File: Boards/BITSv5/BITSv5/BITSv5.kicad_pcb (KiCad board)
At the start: 4 copper layers, 61.7 x 59.5 mm, 82 parts, among them J1 Conn_01x10_Pin, J2 USB_C_Receptacle_USB2.0, J3 Conn_01x07, J4 Conn_01x10_Pin, Q1 Q_NMOS_GSD, Q2 Q_PMOS_GSD, SW1 SW_Push, SW3 SLIDE, U1 MCU_RaspberryPi_RP2040_RP2040, U10 USBLC6-2SC6, U2 W25Q128JVS, U3 MAX-M10S, U4 MAX25255AFDA/VY+, U6 XBee_SMT, U7 TPS2121RUXR, U8 LT6703CDC-3, U9 TVS1800DRVR, Y1 12MHz

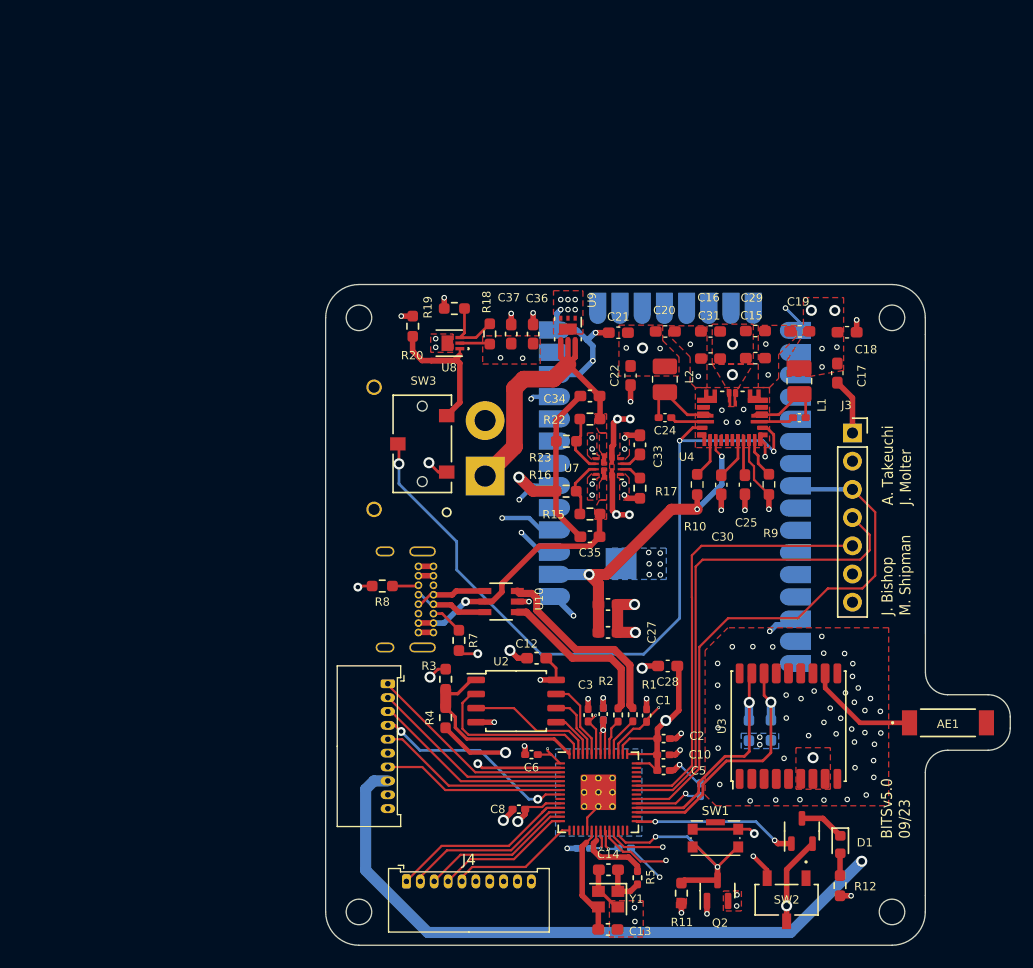
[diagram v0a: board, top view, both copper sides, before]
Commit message: bits v5 w/ dorji radio
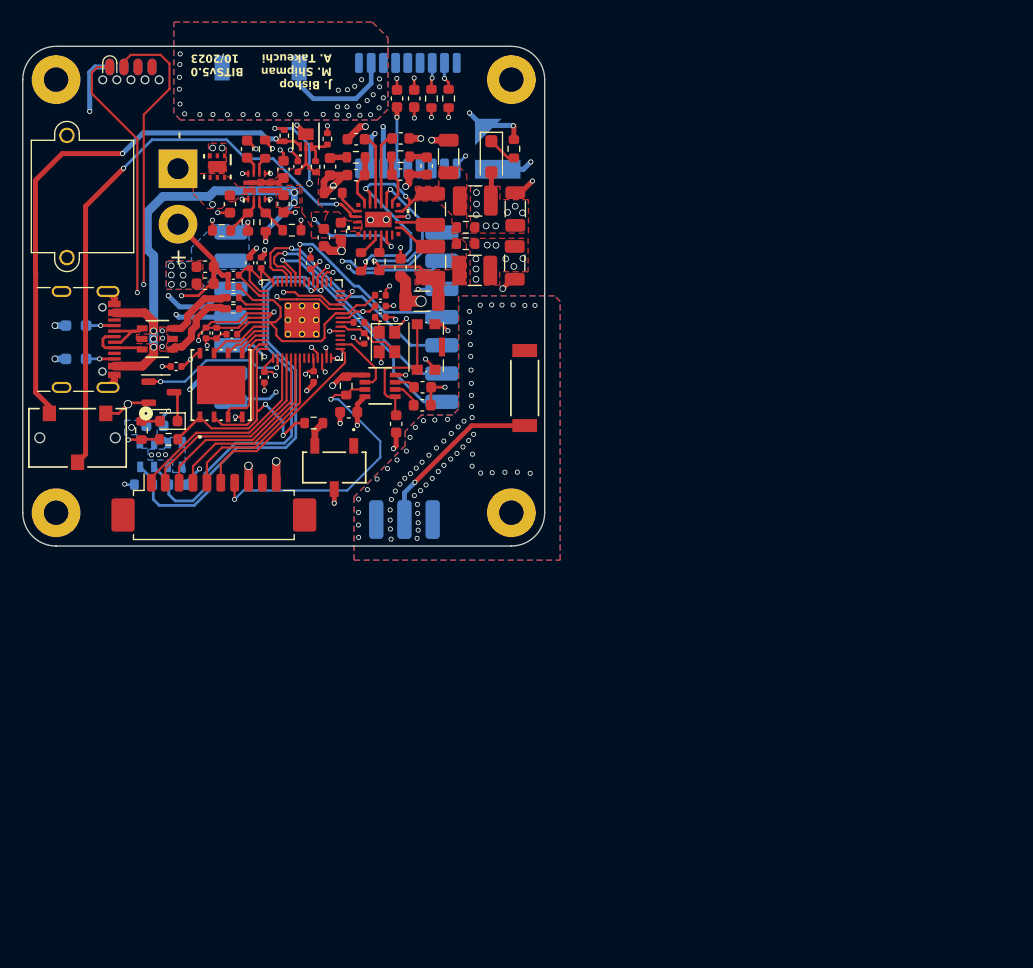
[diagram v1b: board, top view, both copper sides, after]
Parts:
- removed C31: 0.1uF, Capacitor_SMD:C_0603_1608Metric_Pad1.08x0.95mm_HandSolder
- removed J4: Conn_01x10_Pin, Connector_Molex:Molex_PicoBlade_53048-1010_1x10_P1.25mm_Horizontal
- removed Q2: Q_PMOS_GSD, Package_TO_SOT_SMD:SOT-23
- added AE2: Antenna, BITSv5:ANT_0915AT43A0026E_JOT, F.Cu at (150.4, 73.0)
- added BT2: 3V, BITSv5:SEIKO_ML414H_IV01E, B.Cu at (148.7, 51.4)
- added C38: 15uF, Capacitor_SMD:C_1206_3216Metric, F.Cu at (149.5, 61.7)
- added C39: 1uF, Capacitor_SMD:C_0603_1608Metric, F.Cu at (140.5, 46.9)
- added C40: 1uF, Capacitor_SMD:C_0603_1608Metric, F.Cu at (138.9, 46.9)
- added C41: 1uF, Capacitor_SMD:C_0603_1608Metric, F.Cu at (134.6, 75.2)
- added C42: 100nF, Capacitor_SMD:C_0603_1608Metric, F.Cu at (141.2, 74.5)
- added C43: 200nF, Capacitor_SMD:C_0603_1608Metric, F.Cu at (141.2, 72.9)
- added D2: 0.5A/40V/240mV, Diode_SMD:D_SOD-123F, F.Cu at (147.4, 52.1)
- added H1: M2, MountingHole:MountingHole_2.2mm_M2_Pad, F.Cu at (108.2, 45.2)
- added H2: M2, MountingHole:MountingHole_2.2mm_M2_Pad, F.Cu at (108.2, 84.2)
- added H3: M2, MountingHole:MountingHole_2.2mm_M2_Pad, F.Cu at (149.2, 84.2)
- added H4: M2, MountingHole:MountingHole_2.2mm_M2_Pad, F.Cu at (149.2, 45.2)
- added L3: 3.3uH, Inductor_SMD:L_1210_3225Metric, F.Cu at (146.0, 56.1)
- added L4: 3.3uH, Inductor_SMD:L_1210_3225Metric, F.Cu at (145.9, 62.4)
- added R13: 100m, Resistor_SMD:R_0603_1608Metric, F.Cu at (145.1, 60.0)
- added R14: 3.3K, Resistor_SMD:R_0603_1608Metric, F.Cu at (149.4, 51.4)
- added R27: 22.1K, Resistor_SMD:R_0603_1608Metric, F.Cu at (139.2, 52.1)
- added R29: 100K, Resistor_SMD:R_0603_1608Metric, F.Cu at (137.3, 61.6)
- added R32: 34.8K, Resistor_SMD:R_0603_1608Metric, F.Cu at (135.2, 52.2)
- added R33: 100K, Resistor_SMD:R_0603_1608Metric, F.Cu at (135.7, 61.6)
- added R34: 15K, Resistor_SMD:R_0603_1608Metric, F.Cu at (133.2, 55.4)
- added R6: 10K, Resistor_SMD:R_0603_1608Metric, B.Cu at (116.1, 81.7)
- added U11: MS5607-02BA, Package_LGA:LGA-8_3x5mm_P1.25mm, B.Cu at (117.7, 79.0)
- added U5: LT8653SIV-PBF, BITSv5:LT8653SIV-PBF, F.Cu at (137.2, 57.8)
- AE1, R7, R8, U3: moved to B.Cu
- BT1: moved to F.Cu
- C1, C10, C2, C3, C5, C6, C7, C8: footprint Capacitor_SMD:C_0402_1005Metric_Pad0.74x0.62mm_HandSolder -> Capacitor_SMD:C_0402_1005Metric
- C11, C32, C4, C9: footprint Capacitor_SMD:C_0402_1005Metric_Pad0.74x0.62mm_HandSolder -> Capacitor_SMD:C_0402_1005Metric; moved to F.Cu
- C12, C13, C14, C37: footprint Capacitor_SMD:C_0603_1608Metric_Pad1.08x0.95mm_HandSolder -> Capacitor_SMD:C_0402_1005Metric
- C15: value 0.1uF -> 4.7uF; footprint Capacitor_SMD:C_0603_1608Metric_Pad1.08x0.95mm_HandSolder -> Capacitor_SMD:C_0603_1608Metric
- C16: value 4.7uF -> 47uF; footprint Capacitor_SMD:C_0603_1608Metric_Pad1.08x0.95mm_HandSolder -> Capacitor_SMD:C_1206_3216Metric
- C17: value 22uF -> 4.7pF; footprint Capacitor_SMD:C_0603_1608Metric_Pad1.08x0.95mm_HandSolder -> Capacitor_SMD:C_0603_1608Metric
- C18, C21: value 22uF -> 470pF; footprint Capacitor_SMD:C_0603_1608Metric_Pad1.08x0.95mm_HandSolder -> Capacitor_SMD:C_0603_1608Metric
- C19: value 22uF -> 10nF; footprint Capacitor_SMD:C_0603_1608Metric_Pad1.08x0.95mm_HandSolder -> Capacitor_SMD:C_0603_1608Metric
- C20: value 22uF -> 100uF; footprint Capacitor_SMD:C_0603_1608Metric_Pad1.08x0.95mm_HandSolder -> Capacitor_SMD:C_1206_3216Metric
- C22: value 22uF -> 100nF; footprint Capacitor_SMD:C_0603_1608Metric_Pad1.08x0.95mm_HandSolder -> Capacitor_SMD:C_0603_1608Metric
- C23: value 0.1uF -> 4.7pF; footprint Capacitor_SMD:C_0402_1005Metric_Pad0.74x0.62mm_HandSolder -> Capacitor_SMD:C_0603_1608Metric
- C24: value 0.1uF -> 10nF; footprint Capacitor_SMD:C_0402_1005Metric_Pad0.74x0.62mm_HandSolder -> Capacitor_SMD:C_0603_1608Metric
- C25: value 2.2uF -> 1uF; footprint Capacitor_SMD:C_0603_1608Metric_Pad1.08x0.95mm_HandSolder -> Capacitor_SMD:C_0603_1608Metric
- C26: value 100pF -> 10uF; footprint Capacitor_SMD:C_0603_1608Metric_Pad1.08x0.95mm_HandSolder -> Capacitor_SMD:C_0603_1608Metric
- C27, C33, C34, C35, C36: footprint Capacitor_SMD:C_0603_1608Metric_Pad1.08x0.95mm_HandSolder -> Capacitor_SMD:C_0603_1608Metric
- C28: value 10uF -> 15uF; footprint Capacitor_SMD:C_0603_1608Metric_Pad1.08x0.95mm_HandSolder -> Capacitor_SMD:C_1206_3216Metric
- C29: value 4.7uF -> 100nF; footprint Capacitor_SMD:C_0603_1608Metric_Pad1.08x0.95mm_HandSolder -> Capacitor_SMD:C_0603_1608Metric; moved to B.Cu
- C30: value 4.7uF -> 100nF; footprint Capacitor_SMD:C_0603_1608Metric_Pad1.08x0.95mm_HandSolder -> Capacitor_SMD:C_0603_1608Metric
- J1: footprint Connector_Molex:Molex_PicoBlade_53048-1010_1x10_P1.25mm_Horizontal -> Connector_Molex:Molex_PicoBlade_53261-1071_1x10-1MP_P1.25mm_Horizontal
- J2: footprint Connector_USB:USB_C_Receptacle_GCT_USB4085 -> Connector_USB:USB_C_Receptacle_GCT_USB4105-xx-A_16P_TopMnt_Horizontal; moved to F.Cu
- J3: value Conn_01x07 -> SOICbite; footprint Connector_PinSocket_2.54mm:PinSocket_1x07_P2.54mm_Vertical -> BITSv5:SOIC_clipProgSmall
- L1, L2: value 0.47uH -> 2.2uH; footprint Inductor_SMD:L_1008_2520Metric_Pad1.43x2.20mm_HandSolder -> Inductor_SMD:L_1210_3225Metric
- R1, R2: value 27Ω -> 27; footprint Resistor_SMD:R_0402_1005Metric_Pad0.72x0.64mm_HandSolder -> Resistor_SMD:R_0402_1005Metric
- R10: value 10K -> 100m; footprint Resistor_SMD:R_0603_1608Metric_Pad0.98x0.95mm_HandSolder -> Resistor_SMD:R_0603_1608Metric
- R11: value 10K -> 100K; footprint Resistor_SMD:R_0603_1608Metric_Pad0.98x0.95mm_HandSolder -> Resistor_SMD:R_0603_1608Metric
- R12, R15, R16, R22, R23, R4: footprint Resistor_SMD:R_0603_1608Metric_Pad0.98x0.95mm_HandSolder -> Resistor_SMD:R_0603_1608Metric
- R17: value 46.4K -> 44.2K; footprint Resistor_SMD:R_0603_1608Metric_Pad0.98x0.95mm_HandSolder -> Resistor_SMD:R_0603_1608Metric
- R18, R19, R20: footprint Resistor_SMD:R_0603_1608Metric_Pad0.98x0.95mm_HandSolder -> Resistor_SMD:R_0402_1005Metric
- R21, R24: footprint Resistor_SMD:R_0603_1608Metric_Pad0.98x0.95mm_HandSolder -> Resistor_SMD:R_0603_1608Metric; moved to F.Cu
- R3: value 10K -> DNF; footprint Resistor_SMD:R_0603_1608Metric_Pad0.98x0.95mm_HandSolder -> Resistor_SMD:R_0603_1608Metric
- R5: footprint Resistor_SMD:R_0402_1005Metric_Pad0.72x0.64mm_HandSolder -> Capacitor_SMD:C_0402_1005Metric
- R9: footprint Resistor_SMD:R_0603_1608Metric_Pad0.98x0.95mm_HandSolder -> Resistor_SMD:R_0603_1608Metric; moved to B.Cu
- U10: footprint BITSv5:SOT23-6L_STM-M -> BITSv5:SOT23-6L_STM
- U2: footprint Package_SO:SOIC-8_5.23x5.23mm_P1.27mm -> BITSv5:WSON_128JVPIQ_WIN
- U4: value MAX25255AFDA/VY+ -> DRF1262TL; footprint BITSv5:21-100477_90-100168_MXM -> BITSv5:DRF1262TL; moved to B.Cu
- U6: value XBee_SMT -> TPS2121RUXR; footprint BITSv5:XCVR_XBP9X-DMUS-001 -> BITSv5:TPS2121; moved to F.Cu
- U7: value TPS2121RUXR -> MAX6747KA29+T; footprint BITSv5:TPS2121 -> BITSv5:21-0078H_MXM
- moved AE1 85.5 mm to (126.6, 44.2), turned to 180 degrees
- moved R12 75.1 mm to (115.9, 76.8)
- moved J3 73.2 mm to (115.0, 43.3), turned to 180 degrees
- moved D1 71.5 mm to (118.4, 76.0), turned to 180 degrees
- moved Q1 69.9 mm to (117.7, 73.3), turned to 0 degrees
- moved U3 64.8 mm to (139.9, 48.5)
- moved R21 64.6 mm to (142.0, 46.9)
- moved R24 63.0 mm to (143.6, 46.9)
- moved C32 61.8 mm to (126.7, 61.7)
- moved C4 58.3 mm to (124.0, 68.1), turned to 180 degrees
- moved C13 57.6 mm to (136.0, 68.5), turned to -90 degrees
- moved C2 56.9 mm to (124.2, 62.8), turned to 180 degrees
- moved SW2 56.3 mm to (133.3, 80.1)
- moved R5 55.9 mm to (135.5, 67.1), turned to 180 degrees
- moved C8 54.9 mm to (125.7, 61.7), turned to 90 degrees
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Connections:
- net /GPS_SCL renamed /SCL
- net /XOUT renamed Net-(U1-XOUT)
- C13 pad 1: GND -> Net-(U1-XIN)
- C13 pad 2: /XIN -> GND
- C14 pad 1: GND -> Net-(C14-Pad1)
- C14 pad 2: Net-(C14-Pad2) -> GND
- C15 pad 1: GND -> VCC
- C15 pad 2: VCC -> GND
- C16 pad 1: VCC -> Net-(U5-FB1)
- C17 pad 1: GND -> Net-(U5-VC1)
- C17 pad 2: +5V -> GND
- C18 pad 1: GND -> Net-(C18-Pad1)
- C18 pad 2: +5V -> GND
- C19 pad 1: GND -> Net-(U5-SS1)
- C19 pad 2: +5V -> GND
- C20 pad 1: GND -> Net-(U5-BIAS)
- C20 pad 2: +3V3 -> GND
- C21 pad 1: GND -> Net-(C21-Pad1)
- C21 pad 2: +3V3 -> GND
- C22 pad 1: GND -> VCC
- C22 pad 2: +3V3 -> GND
- C23 pad 1: Net-(U4-BST2) -> Net-(U5-VC2)
- C23 pad 2: Net-(U4-LX2) -> GND
- C24 pad 1: Net-(U4-BST1) -> Net-(U5-SS2)
- C24 pad 2: Net-(U4-LX1) -> GND
- C25 pad 1: GND -> Net-(U5-VCC)
- C25 pad 2: Net-(U4-EXTVCC) -> GND
- C26 pad 1: +3V3 -> +5V
- C27 pad 1: +3V3 -> +5V
- C29 pad 1: GND -> +3V3
- C29 pad 2: VCC -> GND
- C30 pad 1: GND -> Net-(U7-*MR)
- C30 pad 2: Net-(U4-BIAS) -> GND
- C33 pad 1: Net-(U7-SS) -> Net-(U6-SS)
- J1 pad 7: /IRIDIUM_ON/OFF -> /RESET
- J3 pad 1: GND -> /RP_SWCLK
- J3 pad 2: /XBEE_DTR -> /RP_SWD
- J3 pad 3: /XBEE_RTS -> unconnected-(J3-Pin_3-Pad3)
- J3 pad 4: /XBEE_DIN -> unconnected-(J3-Pin_4-Pad4)
- J3 pad 5: /XBEE_DOUT -> unconnected-(J3-Pin_5-Pad5)
- J3 pad 6: /RP_SWD -> unconnected-(J3-Pin_6-Pad6)
- J3 pad 7: /RP_SWCLK -> unconnected-(J3-Pin_7-Pad7)
- L1 pad 1: +5V -> Net-(U5-FB1)
- L1 pad 2: Net-(U4-LX2) -> Net-(U5-SW1)
- L2 pad 1: Net-(U4-LX1) -> Net-(U5-BIAS)
- L2 pad 2: +3V3 -> Net-(U5-SW2)
- R10 pad 2: Net-(U4-PGOOD1) -> Net-(U5-BIAS)
- R11 pad 2: Net-(Q2-D) -> /RESET
- R15 pad 2: Net-(U7-OV1) -> Net-(U6-OV1)
- R16 pad 1: Net-(U7-OV1) -> Net-(U6-OV1)
- R17 pad 1: Net-(U7-ILM) -> Net-(U6-ILM)
- R21 pad 2: /GPS_SDA -> /SDA
- R22 pad 2: Net-(U7-OV2) -> Net-(U6-OV2)
- R23 pad 1: Net-(U7-OV2) -> Net-(U6-OV2)
- R5 pad 1: Net-(C14-Pad2) -> Net-(C14-Pad1)
- R9 pad 1: +5V -> +3V3
- R9 pad 2: Net-(U4-PGOOD2) -> /SDA
- SW1 pad 2: Net-(Q2-D) -> Net-(U7-*MR)
- U1 pad 11: /2.4_MISO -> /DRF_TXEN
- U1 pad 12: /2.4_SSEL -> /DRF_SW
- U1 pad 13: /2.4_SCLK -> /DRF_DIO1
- U1 pad 14: /2.4_MOSI -> /DRF_BUSY
- U1 pad 15: /2.4_ATTN -> /IRIDIUM_TXD
- U1 pad 16: unconnected-(U1-GPIO13-Pad16) -> /WATCHDOG
- U1 pad 2: /IRIDIUM_TXD -> /LED
- U1 pad 20: /XIN -> Net-(U1-XIN)
- U1 pad 26: Net-(Q2-D) -> /RESET
- U1 pad 29: /LED -> unconnected-(U1-GPIO18-Pad29)
- U1 pad 31: /GPS_SDA -> /SDA
- U1 pad 34: /XBEE_RTS -> unconnected-(U1-GPIO22-Pad34)
- U1 pad 36: /XBEE_DIN -> /DRF_MISO
- U1 pad 37: /XBEE_DOUT -> /DRF_CS
- U1 pad 38: unconnected-(U1-GPIO26_ADC0-Pad38) -> /DRF_CLK
- U1 pad 39: unconnected-(U1-GPIO27_ADC1-Pad39) -> /DRF_MOSI
- U1 pad 40: /VBAT -> unconnected-(U1-GPIO28_ADC2-Pad40)
- U1 pad 6: /IRIDIUM_RING -> /IRIDIUM_NETAV
- U1 pad 7: /IRIDIUM_ON/OFF -> /IRIDIUM_RING
- U1 pad 8: /IRIDIUM_NETAV -> unconnected-(U1-GPIO6-Pad8)
- U3 pad 16: /GPS_SDA -> /SDA
- U3 pad 6: +3V3 -> Net-(BT2-+)
- U4 pad 1: +3V3 -> /DRF_SW
- U4 pad 10: unconnected-(U4-NC-Pad10) -> /RESET
- U4 pad 11: Net-(U4-LX1) -> /DRF_MISO
- U4 pad 12: Net-(U4-BST1) -> /DRF_MOSI
- U4 pad 13: /LVC_CUTOFF -> /DRF_CLK
- U4 pad 14: unconnected-(U4-SYNCOUT-Pad14) -> /DRF_CS
- U4 pad 15: Net-(U4-PGOOD1) -> GND
- U4 pad 16: +3V3 -> Net-(AE2-A)
- U4 pad 17: unconnected-(U4-TEMP-Pad17) -> GND
- U4 pad 2: /LVC_CUTOFF -> GND
- U4 pad 3: Net-(U4-BST2) -> /DRF_TXEN
- U4 pad 4: Net-(U4-LX2) -> GND
- U4 pad 5: unconnected-(U4-NC-Pad5) -> GND
- U4 pad 6: GND -> +5V
- U4 pad 7: VCC -> +5V
- U4 pad 8: VCC -> /DRF_DIO1
- U4 pad 9: GND -> /DRF_BUSY
- U6 pad 1: GND -> VCC
- U6 pad 10: /XBEE_DTR -> Net-(U6-ILM)
- U6 pad 11: GND -> Net-(U6-SS)
- U6 pad 12: unconnected-(U6-DO19/~{SPI_ATTN}-Pad12) -> GND
- U6 pad 2: +3V3 -> +BATT
- U6 pad 3: /XBEE_DOUT -> GND
- U6 pad 4: /XBEE_DIN -> Net-(U6-OV2)
- U6 pad 5: unconnected-(U6-DIO12-Pad5) -> Net-(U6-OV1)
- U6 pad 6: /XBEE_RESET -> GND
- U6 pad 7: unconnected-(U6-DIO10/RSSI/PWM0-Pad7) -> VBUS
- U6 pad 8: unconnected-(U6-DIO11/PWM1-Pad8) -> VCC
- U6 pad 9: (no net) -> GND
- U7 pad 1: VCC -> Net-(U7-*MR)
- U7 pad 2: +BATT -> Net-(U7-SWT)
- U7 pad 3: GND -> Net-(U7-SRT)
- U7 pad 4: Net-(U7-OV2) -> GND
- U7 pad 5: Net-(U7-OV1) -> +3V3
- U7 pad 6: GND -> /WATCHDOG
- U7 pad 7: VBUS -> /RESET
- U7 pad 8: VCC -> +3V3
- Y1 pad 1: Net-(C14-Pad2) -> Net-(C14-Pad1)
- Y1 pad 3: /XIN -> Net-(U1-XIN)
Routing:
- net /XBEE_RESET: track 86.1 -> 0.00 mm, vias 2 -> 0
- net /XBEE_DIN: track 81.7 -> 0.00 mm, vias 1 -> 0
- net /XBEE_DOUT: track 73.7 -> 0.00 mm, vias 1 -> 0
- net /SDA: track 0.00 -> 70.9 mm, vias 0 -> 3
- net Net-(SW2-B): track 61.7 -> 2.36 mm, vias 2 -> 0
- net /XBEE_RTS: track 49.1 -> 0.00 mm
- net /SCL: track 21.5 -> 69.9 mm, vias 1 -> 3
- net /RESET: track 0.00 -> 47.2 mm, vias 0 -> 4
- net /XBEE_DTR: track 36.4 -> 0.00 mm, vias 1 -> 0
- net +5V: track 66.2 -> 34.9 mm, vias 7 -> 15
- net Net-(SW3-C): track 17.3 -> 47.6 mm, vias 0 -> 2
- net /GPS_SDA: track 23.9 -> 0.00 mm, vias 1 -> 0
- net +BATT: track 28.0 -> 4.67 mm, vias 0 -> 2
- net /DRF_CS: track 0.00 -> 22.9 mm, vias 0 -> 1
- net /DRF_MOSI: track 0.00 -> 22.9 mm, vias 0 -> 1
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- added copper zone on B.Cu, net +5V
- added copper zone on F.Cu, net Net-(U5-BIAS)
- added copper zone on F.Cu, net Net-(U5-FB1)
- removed copper zone on In2.Cu, net VCC
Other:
- board size 61.7 x 59.5 mm -> 47 x 45 mm
- board text added: "BITSv5.0 10/2023"
- board text added: "J. Bishop M. Shipman A. Takeuchi"
- board text removed: "A. Takeuchi J. Molter"
- board text removed: "BITSv5.0 09/23"
- board text removed: "J. Bishop M. Shipman"
